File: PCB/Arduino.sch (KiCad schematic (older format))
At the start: 1 part, among them U2 MCU-ATMEGA328P-AU(TQFP32)

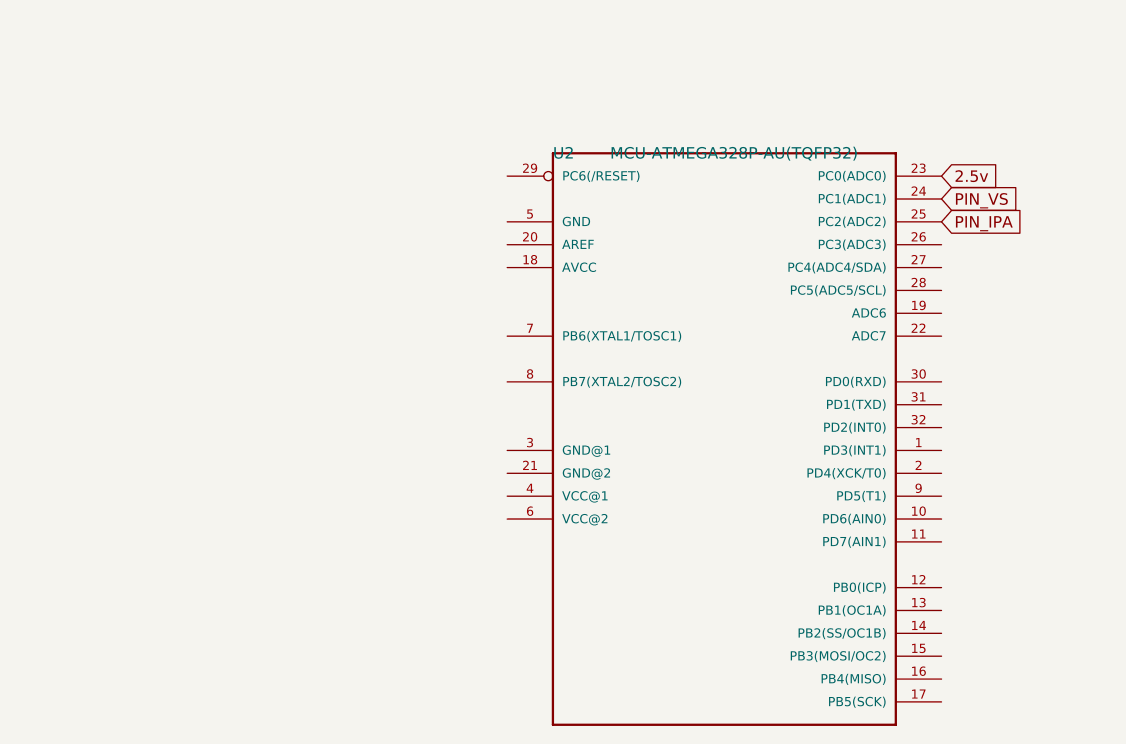
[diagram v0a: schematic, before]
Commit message: -
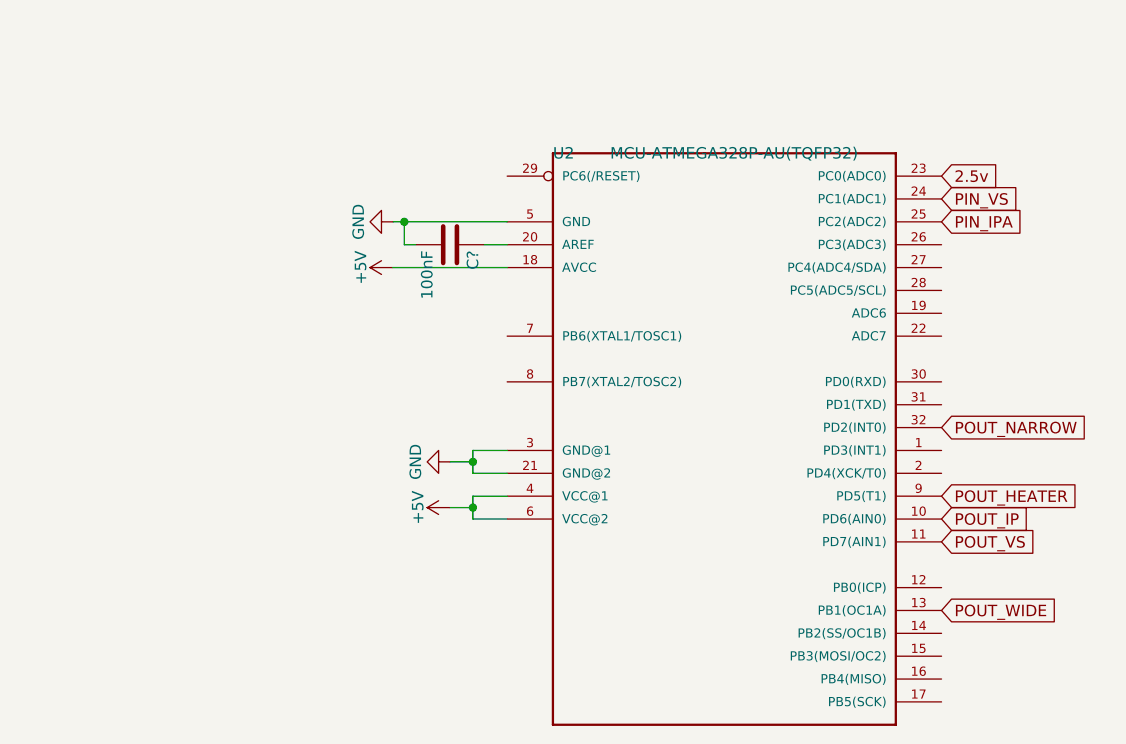
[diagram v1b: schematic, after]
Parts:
- added C?: 100nF, symbol 100nF
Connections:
- net POUT_IP: now reaches U2.10 (PD6(AIN0))
- net POUT_VS: now reaches U2.11 (PD7(AIN1))
- net POUT_WIDE: now reaches U2.13 (PB1(OC1A))
- net +5V: now reaches U2.18 (AVCC)
- net +5V: now also U2.4 (VCC@1), U2.6 (VCC@2)
- net at U2.20 (AREF): now also C?.1
- net GND: now reaches U2.21 (GND@2)
- net GND: now also U2.3 (GND@1), U2.5 (GND), C?.2
- net POUT_NARROW: now reaches U2.32 (PD2(INT0))
- net POUT_HEATER: now reaches U2.9 (PD5(T1))
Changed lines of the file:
@@
 Text GLabel 6250 2800 2    50   Input ~ 0
 PIN_IPA
+Text GLabel 6250 3700 2    50   Input ~ 0
+POUT_NARROW
+Text GLabel 6250 4000 2    50   Input ~ 0
+POUT_HEATER
+Text GLabel 6250 4100 2    50   Input ~ 0
+POUT_IP
+Text GLabel 6250 4200 2    50   Input ~ 0
+POUT_VS
+Text GLabel 6250 4500 2    50   Input ~ 0
+POUT_WIDE
+$Comp
+L +5V #PWR?
+U 1 1 55FC7481
+P 4100 4050
+F 0 "#PWR?" H 4100 3900 50  0001 C CNN
+F 1 "+5V" H 4100 4190 50  0000 C CNN
+F 2 "" H 4100 4050 60  0000 C CNN
+F 3 "" H 4100 4050 60  0000 C CNN
+	1    4100 4050
+	0    -1   -1   0
+$EndComp
+Wire Wire Line
+	4350 4000 4200 4000
+Wire Wire Line
+	4200 4000 4200 4100
+Wire Wire Line
+	4200 4100 4350 4100
+Wire Wire Line
+	4200 4050 4100 4050
+Connection ~ 4200 4050
+$Comp
+L GND #PWR?
+U 1 1 55FC752E
+P 3850 2800
+F 0 "#PWR?" H 3850 2550 50  0001 C CNN
+F 1 "GND" H 3850 2650 50  0000 C CNN
+F 2 "" H 3850 2800 60  0000 C CNN
+F 3 "" H 3850 2800 60  0000 C CNN
+	1    3850 2800
+	0    1    1    0
+$EndComp
+Wire Wire Line
+	4350 2800 3850 2800
+$Comp
+L +5V #PWR?
+U 1 1 55FC754C
+P 3850 3000
+F 0 "#PWR?" H 3850 2850 50  0001 C CNN
+F 1 "+5V" H 3850 3140 50  0000 C CNN
+F 2 "" H 3850 3000 60  0000 C CNN
+F 3 "" H 3850 3000 60  0000 C CNN
+	1    3850 3000
+	0    -1   -1   0
+$EndComp
+Wire Wire Line
+	4350 3000 3850 3000
+$Comp
+L 100nF C?
+U 1 1 55FC756B
+P 4100 2900
+F 0 "C?" H 4125 3000 50  0000 L CNN
+F 1 "100nF" H 4125 2800 50  0000 L CNN
+F 2 "" H 4138 2750 30  0000 C CNN
+F 3 "" H 4100 2900 60  0000 C CNN
+F 4 "311-1344-1-ND" V 4280 3000 60  0001 C CNN "Ref Digikey"
+	1    4100 2900
+	0    1    1    0
+$EndComp
+Wire Wire Line
+	4350 2900 4250 2900
+Wire Wire Line
+	3950 2900 3900 2900
+Wire Wire Line
+	3900 2900 3900 2800
+Connection ~ 3900 2800
+$Comp
+L GND #PWR?
+U 1 1 55FC7632
+P 4100 3850
+F 0 "#PWR?" H 4100 3600 50  0001 C CNN
+F 1 "GND" H 4100 3700 50  0000 C CNN
+F 2 "" H 4100 3850 60  0000 C CNN
+F 3 "" H 4100 3850 60  0000 C CNN
+	1    4100 3850
+	0    1    1    0
+$EndComp
+Wire Wire Line
+	4350 3800 4200 3800
+Wire Wire Line
+	4200 3800 4200 3900
+Wire Wire Line
+	4200 3900 4350 3900
+Wire Wire Line
+	4200 3850 4100 3850
+Connection ~ 4200 3850
 $EndSCHEMATC

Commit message: - routage
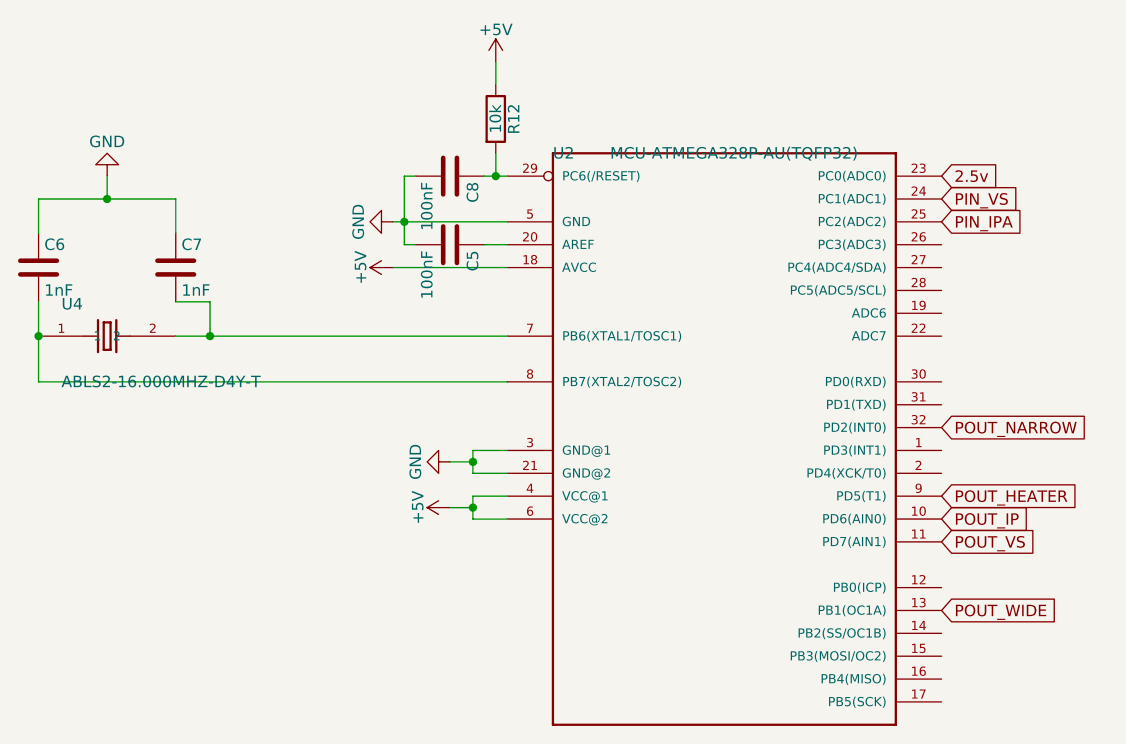
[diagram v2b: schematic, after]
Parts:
- added C6, C7: 1nF, condensateurs:C_0603_HandSoldering, symbol 1nF
- added C8: 100nF, condensateurs:C_0603_HandSoldering, symbol 100nF
- added R12: 10k, resistances:R_0603_HandSoldering, symbol 10k
- added U4: ABLS2-16.000MHZ-D4Y-T, Quartz:HC-49, symbol ABLS2-8.000MHZ-D4Y-T
- C5: renamed from C?; footprint (none) -> condensateurs:C_0603_HandSoldering
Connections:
- net +5V: now also R12.1
- net GND: now also C6.1, C7.1, C8.2
- net at U2.29 (PC6(/RESET)): now also C8.1, R12.2
- net at U2.7 (PB6(XTAL1/TOSC1)): now also C7.2, U4.2
- net at U2.8 (PB7(XTAL2/TOSC2)): now also C6.2, U4.1
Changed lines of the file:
@@
 EESchema Schematic File Version 2
-LIBS:TLV2252AID
 LIBS:Power
 LIBS:Resistances_SMD_0603
@@
 LIBS:Microcontroleur_Atmel_SMD_TQFP
 LIBS:Barrettes_TH
+LIBS:Amplificateur_Operationel_SMD_SOIC
+LIBS:Quartz_SMD
+LIBS:Regulateurs_SMD_SOT89
+LIBS:Regulateurs_SMD_SOT23
 LIBS:LO2SC-cache
 EELAYER 25 0
@@
 POUT_WIDE
 $Comp
-L +5V #PWR?
+L +5V #PWR06
 U 1 1 55FC7481
 P 4100 4050
-F 0 "#PWR?" H 4100 3900 50  0001 C CNN
+F 0 "#PWR06" H 4100 3900 50  0001 C CNN
 F 1 "+5V" H 4100 4190 50  0000 C CNN
 F 2 "" H 4100 4050 60  0000 C CNN
@@
 Connection ~ 4200 4050
 $Comp
-L GND #PWR?
+L GND #PWR07
 U 1 1 55FC752E
 P 3850 2800
-F 0 "#PWR?" H 3850 2550 50  0001 C CNN
+F 0 "#PWR07" H 3850 2550 50  0001 C CNN
 F 1 "GND" H 3850 2650 50  0000 C CNN
 F 2 "" H 3850 2800 60  0000 C CNN
@@
 $EndComp
 Wire Wire Line
-	4350 2800 3850 2800
-$Comp
-L +5V #PWR?
+	3850 2800 4350 2800
+$Comp
+L +5V #PWR08
 U 1 1 55FC754C
 P 3850 3000
-F 0 "#PWR?" H 3850 2850 50  0001 C CNN
+F 0 "#PWR08" H 3850 2850 50  0001 C CNN
 F 1 "+5V" H 3850 3140 50  0000 C CNN
 F 2 "" H 3850 3000 60  0000 C CNN
@@
 	4350 3000 3850 3000
 $Comp
-L 100nF C?
+L 100nF C5
 U 1 1 55FC756B
 P 4100 2900
-F 0 "C?" H 4125 3000 50  0000 L CNN
+F 0 "C5" H 4125 3000 50  0000 L CNN
 F 1 "100nF" H 4125 2800 50  0000 L CNN
-F 2 "" H 4138 2750 30  0000 C CNN
+F 2 "condensateurs:C_0603_HandSoldering" H 4138 2750 30  0001 C CNN
 F 3 "" H 4100 2900 60  0000 C CNN
 F 4 "311-1344-1-ND" V 4280 3000 60  0001 C CNN "Ref Digikey"
@@
 	4350 2900 4250 2900
 Wire Wire Line
-	3950 2900 3900 2900
-Wire Wire Line
-	3900 2900 3900 2800
+	3900 2900 3950 2900
+Wire Wire Line
+	3900 2600 3900 2900
 Connection ~ 3900 2800
 $Comp
-L GND #PWR?
+L GND #PWR09
 U 1 1 55FC7632
 P 4100 3850
-F 0 "#PWR?" H 4100 3600 50  0001 C CNN
+F 0 "#PWR09" H 4100 3600 50  0001 C CNN
 F 1 "GND" H 4100 3700 50  0000 C CNN
 F 2 "" H 4100 3850 60  0000 C CNN
@@
 	4200 3850 4100 3850
 Connection ~ 4200 3850
+$Comp
+L ABLS2-8.000MHZ-D4Y-T U4
+U 1 1 5601374A
+P 2600 3300
+F 0 "U4" H 2400 3440 50  0000 L CNN
+F 1 "ABLS2-16.000MHZ-D4Y-T" H 2400 3100 50  0000 L CNN
+F 2 "Quartz:HC-49" H 2600 3300 50  0001 L CNN
+F 3 "" H 2600 3300 60  0000 C CNN
+	1    2600 3300
+	1    0    0    -1
+$EndComp
+Wire Wire Line
+	2900 3300 4350 3300
+Wire Wire Line
+	2300 3500 4350 3500
+Wire Wire Line
+	2300 3150 2300 3500
+$Comp
+L 1nF C6
+U 1 1 560137E4
+P 2300 3000
+F 0 "C6" H 2325 3100 50  0000 L CNN
+F 1 "1nF" H 2325 2900 50  0000 L CNN
+F 2 "condensateurs:C_0603_HandSoldering" H 2338 2850 30  0001 C CNN
+F 3 "" H 2300 3000 60  0000 C CNN
+F 4 "311-1080-1-ND" V 2480 3100 60  0001 C CNN "Ref Digikey"
+	1    2300 3000
+	1    0    0    -1
+$EndComp
+$Comp
+L 1nF C7
+U 1 1 5601383A
+P 2900 3000
+F 0 "C7" H 2925 3100 50  0000 L CNN
+F 1 "1nF" H 2925 2900 50  0000 L CNN
+F 2 "condensateurs:C_0603_HandSoldering" H 2938 2850 30  0001 C CNN
+F 3 "" H 2900 3000 60  0000 C CNN
+F 4 "311-1080-1-ND" V 3080 3100 60  0001 C CNN "Ref Digikey"
+	1    2900 3000
+	1    0    0    -1
+$EndComp
+$Comp
+L GND #PWR010
+U 1 1 5601389E
+P 2600 2600
+F 0 "#PWR010" H 2600 2350 50  0001 C CNN
+F 1 "GND" H 2600 2450 50  0000 C CNN
+F 2 "" H 2600 2600 60  0000 C CNN
+F 3 "" H 2600 2600 60  0000 C CNN
+	1    2600 2600
+	-1   0    0    1
+$EndComp
+Wire Wire Line
+	2900 2700 2900 2850
+Wire Wire Line
+	2300 2700 2900 2700
+Wire Wire Line
+	2300 2700 2300 2850
+Wire Wire Line
+	2600 2700 2600 2600
+Connection ~ 2600 2700
+Connection ~ 2300 3300
+Wire Wire Line
+	2900 3150 3050 3150
+Wire Wire Line
+	3050 3150 3050 3300
+Connection ~ 3050 3300
+$Comp
+L 100nF C8
+U 1 1 56013DD7
+P 4100 2600
+F 0 "C8" H 4125 2700 50  0000 L CNN
+F 1 "100nF" H 4125 2500 50  0000 L CNN
+F 2 "condensateurs:C_0603_HandSoldering" H 4138 2450 30  0001 C CNN
+F 3 "" H 4100 2600 60  0000 C CNN
+F 4 "311-1344-1-ND" V 4280 2700 60  0001 C CNN "Ref Digikey"
+	1    4100 2600
+	0    1    1    0
+$EndComp
+Wire Wire Line
+	4350 2600 4250 2600
+Wire Wire Line
+	3900 2600 3950 2600
+$Comp
+L 10k R12
+U 1 1 56013ED3
+P 4300 2350
+F 0 "R12" V 4380 2350 50  0000 C CNN
+F 1 "10k" V 4300 2350 50  0000 C CNN
+F 2 "resistances:R_0603_HandSoldering" V 4230 2350 30  0001 C CNN
+F 3 "" V 4380 2350 30  0000 C CNN
+F 4 "311-10kGRCT-ND" V 4480 2450 60  0001 C CNN "Ref Digikey"
+	1    4300 2350
+	1    0    0    -1
+$EndComp
+$Comp
+L +5V #PWR011
+U 1 1 56013F29
+P 4300 2100
+F 0 "#PWR011" H 4300 1950 50  0001 C CNN
+F 1 "+5V" H 4300 2240 50  0000 C CNN
+F 2 "" H 4300 2100 60  0000 C CNN
+F 3 "" H 4300 2100 60  0000 C CNN
+	1    4300 2100
+	1    0    0    -1
+$EndComp
+Wire Wire Line
+	4300 2600 4300 2500
+Connection ~ 4300 2600
+Wire Wire Line
+	4300 2200 4300 2100
 $EndSCHEMATC

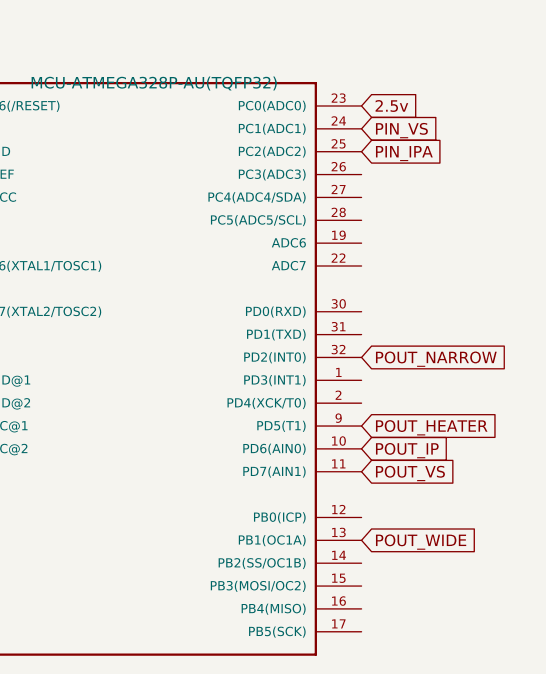
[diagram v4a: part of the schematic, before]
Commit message: ?
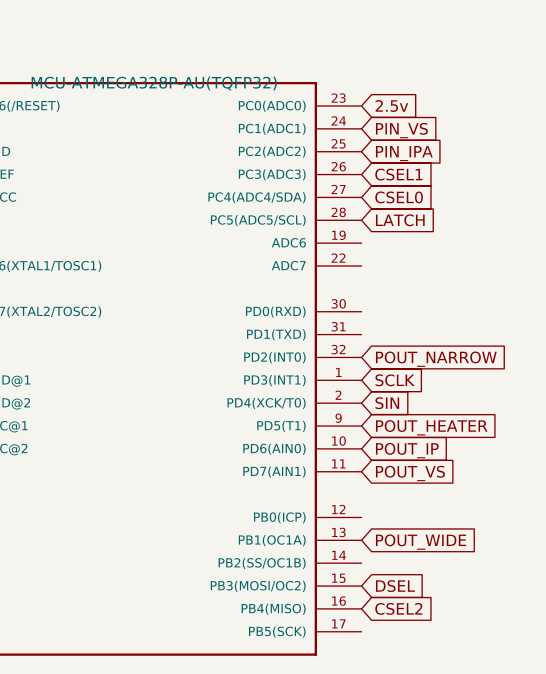
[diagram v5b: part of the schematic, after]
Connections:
- net SCLK: now reaches U2.1 (PD3(INT1))
- net DSEL: now reaches U2.15 (PB3(MOSI/OC2))
- net CSEL2: now reaches U2.16 (PB4(MISO))
- net SIN: now reaches U2.2 (PD4(XCK/T0))
- net CSEL1: now reaches U2.26 (PC3(ADC3))
- net CSEL0: now reaches U2.27 (PC4(ADC4/SDA))
- net LATCH: now reaches U2.28 (PC5(ADC5/SCL))
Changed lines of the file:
@@
 POUT_WIDE
 $Comp
-L +5V #PWR06
+L +5V #PWR010
 U 1 1 55FC7481
 P 4100 4050
-F 0 "#PWR06" H 4100 3900 50  0001 C CNN
+F 0 "#PWR010" H 4100 3900 50  0001 C CNN
 F 1 "+5V" H 4100 4190 50  0000 C CNN
 F 2 "" H 4100 4050 60  0000 C CNN
@@
 Connection ~ 4200 4050
 $Comp
-L GND #PWR07
+L GND #PWR011
 U 1 1 55FC752E
 P 3850 2800
-F 0 "#PWR07" H 3850 2550 50  0001 C CNN
+F 0 "#PWR011" H 3850 2550 50  0001 C CNN
 F 1 "GND" H 3850 2650 50  0000 C CNN
 F 2 "" H 3850 2800 60  0000 C CNN
@@
 	3850 2800 4350 2800
 $Comp
-L +5V #PWR08
+L +5V #PWR012
 U 1 1 55FC754C
 P 3850 3000
-F 0 "#PWR08" H 3850 2850 50  0001 C CNN
+F 0 "#PWR012" H 3850 2850 50  0001 C CNN
 F 1 "+5V" H 3850 3140 50  0000 C CNN
 F 2 "" H 3850 3000 60  0000 C CNN
@@
 Connection ~ 3900 2800
 $Comp
-L GND #PWR09
+L GND #PWR013
 U 1 1 55FC7632
 P 4100 3850
-F 0 "#PWR09" H 4100 3600 50  0001 C CNN
+F 0 "#PWR013" H 4100 3600 50  0001 C CNN
 F 1 "GND" H 4100 3700 50  0000 C CNN
 F 2 "" H 4100 3850 60  0000 C CNN
@@
 $EndComp
 $Comp
-L GND #PWR010
+L GND #PWR014
 U 1 1 5601389E
 P 2600 2600
-F 0 "#PWR010" H 2600 2350 50  0001 C CNN
+F 0 "#PWR014" H 2600 2350 50  0001 C CNN
 F 1 "GND" H 2600 2450 50  0000 C CNN
 F 2 "" H 2600 2600 60  0000 C CNN
@@
 $EndComp
 $Comp
-L +5V #PWR011
+L +5V #PWR015
 U 1 1 56013F29
 P 4300 2100
-F 0 "#PWR011" H 4300 1950 50  0001 C CNN
+F 0 "#PWR015" H 4300 1950 50  0001 C CNN
 F 1 "+5V" H 4300 2240 50  0000 C CNN
 F 2 "" H 4300 2100 60  0000 C CNN
@@
 Wire Wire Line
 	4300 2200 4300 2100
+Text GLabel 6250 4800 2    50   Input ~ 0
+CSEL2
+Text GLabel 6250 4700 2    50   Input ~ 0
+DSEL
+Text GLabel 6250 3800 2    50   Input ~ 0
+SCLK
+Text GLabel 6250 3900 2    50   Input ~ 0
+SIN
+Text GLabel 6250 2900 2    50   Input ~ 0
+CSEL1
+Text GLabel 6250 3000 2    50   Input ~ 0
+CSEL0
+Text GLabel 6250 3100 2    50   Input ~ 0
+LATCH
 $EndSCHEMATC
